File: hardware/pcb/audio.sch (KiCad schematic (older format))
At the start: 23 parts, among them J300 Conn_01x02, J301 AudioJack3_Ground_SwitchTR, U300 WM8960

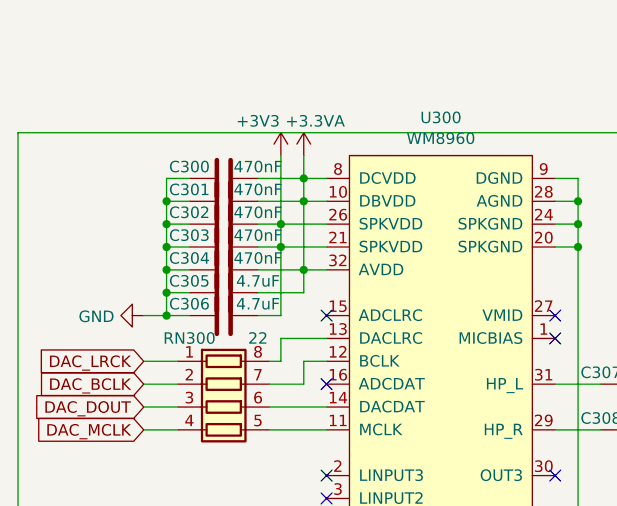
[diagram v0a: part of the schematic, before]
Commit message: vbh: pcb layout
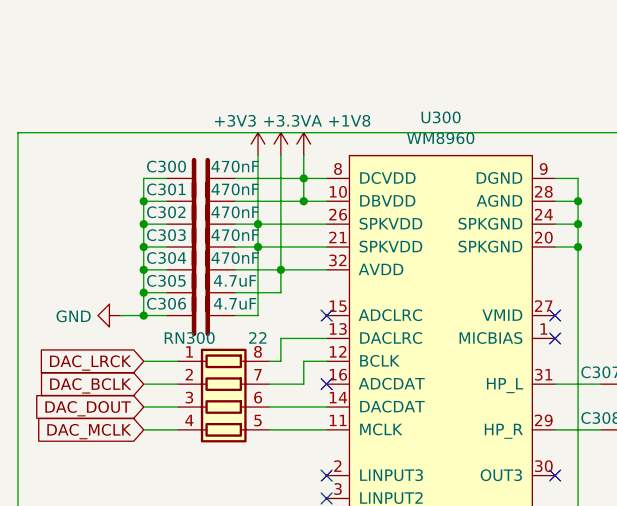
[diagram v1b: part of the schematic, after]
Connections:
- net +3.3VA: no longer C300.1, C301.1, U300.10 (DBVDD), U300.8 (DCVDD)
- new net +1V8: C300.1, C301.1, U300.10 (DBVDD), U300.8 (DCVDD)
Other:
- moved on the sheet: C300, C301, C302, C303, C304, C305, C306
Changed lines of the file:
@@
 L Device:C C?
 U 1 1 5EC1BEE7
-P 4600 3000
+P 4500 3000
 AR Path="/5E1291BC/5EC1BEE7" Ref="C?"  Part="1"
 AR Path="/5E1292AC/5EC1BEE7" Ref="C300"  Part="1"
-F 0 "C300" V 4550 2850 50  0000 C CNN
-F 1 "470nF" V 4550 3150 50  0000 C CNN
-F 2 "Capacitor_SMD:C_0402_1005Metric" H 4638 2850 50  0001 C CNN
-F 3 "~" H 4600 3000 50  0001 C CNN
-	1    4600 3000
+F 0 "C300" V 4450 2850 50  0000 C CNN
+F 1 "470nF" V 4450 3150 50  0000 C CNN
+F 2 "Capacitor_SMD:C_0402_1005Metric" H 4538 2850 50  0001 C CNN
+F 3 "~" H 4500 3000 50  0001 C CNN
+	1    4500 3000
 	0    1    1    0
 $EndComp
@@
 L Device:C C?
 U 1 1 5EC1BEED
-P 4600 3100
+P 4500 3100
 AR Path="/5E1291BC/5EC1BEED" Ref="C?"  Part="1"
 AR Path="/5E1292AC/5EC1BEED" Ref="C301"  Part="1"
-F 0 "C301" V 4550 2950 50  0000 C CNN
-F 1 "470nF" V 4550 3250 50  0000 C CNN
-F 2 "Capacitor_SMD:C_0402_1005Metric" H 4638 2950 50  0001 C CNN
-F 3 "~" H 4600 3100 50  0001 C CNN
-	1    4600 3100
+F 0 "C301" V 4450 2950 50  0000 C CNN
+F 1 "470nF" V 4450 3250 50  0000 C CNN
+F 2 "Capacitor_SMD:C_0402_1005Metric" H 4538 2950 50  0001 C CNN
+F 3 "~" H 4500 3100 50  0001 C CNN
+	1    4500 3100
 	0    1    1    0
 $EndComp
@@
 L Device:C C?
 U 1 1 5EC1BEF3
-P 4600 3500
+P 4500 3500
 AR Path="/5E1291BC/5EC1BEF3" Ref="C?"  Part="1"
 AR Path="/5E1292AC/5EC1BEF3" Ref="C305"  Part="1"
-F 0 "C305" V 4550 3350 50  0000 C CNN
-F 1 "4.7uF" V 4550 3650 50  0000 C CNN
-F 2 "Capacitor_SMD:C_0603_1608Metric" H 4638 3350 50  0001 C CNN
-F 3 "~" H 4600 3500 50  0001 C CNN
-	1    4600 3500
-	0    1    1    0
-$EndComp
-Wire Wire Line
-	4450 3000 4350 3000
-Wire Wire Line
-	4350 3000 4350 3100
-Wire Wire Line
-	4450 3100 4350 3100
-Connection ~ 4350 3100
-Wire Wire Line
-	4350 3100 4350 3200
-Wire Wire Line
-	4450 3200 4350 3200
-Connection ~ 4350 3200
+F 0 "C305" V 4450 3350 50  0000 C CNN
+F 1 "4.7uF" V 4450 3650 50  0000 C CNN
+F 2 "Capacitor_SMD:C_0603_1608Metric" H 4538 3350 50  0001 C CNN
+F 3 "~" H 4500 3500 50  0001 C CNN
+	1    4500 3500
+	0    1    1    0
+$EndComp
+Wire Wire Line
+	4350 3000 4250 3000
+Wire Wire Line
+	4250 3000 4250 3100
+Wire Wire Line
+	4350 3100 4250 3100
+Connection ~ 4250 3100
+Wire Wire Line
+	4250 3100 4250 3200
+Wire Wire Line
+	4350 3200 4250 3200
+Connection ~ 4250 3200
 $Comp
 L power:GND #PWR?
 U 1 1 5EC1BEFF
-P 4250 3600
+P 4150 3600
 AR Path="/5E1291BC/5EC1BEFF" Ref="#PWR?"  Part="1"
 AR Path="/5E1292AC/5EC1BEFF" Ref="#PWR055"  Part="1"
-F 0 "#PWR055" H 4250 3350 50  0001 C CNN
-F 1 "GND" V 4255 3472 50  0000 R CNN
-F 2 "" H 4250 3600 50  0001 C CNN
-F 3 "" H 4250 3600 50  0001 C CNN
-	1    4250 3600
+F 0 "#PWR055" H 4150 3350 50  0001 C CNN
+F 1 "GND" V 4155 3472 50  0000 R CNN
+F 2 "" H 4150 3600 50  0001 C CNN
+F 3 "" H 4150 3600 50  0001 C CNN
+	1    4150 3600
 	0    1    1    0
 $EndComp
@@
 L Device:C C?
 U 1 1 5EC1D61E
-P 4600 3600
+P 4500 3600
 AR Path="/5E1291BC/5EC1D61E" Ref="C?"  Part="1"
 AR Path="/5E1292AC/5EC1D61E" Ref="C306"  Part="1"
-F 0 "C306" V 4550 3450 50  0000 C CNN
-F 1 "4.7uF" V 4550 3750 50  0000 C CNN
-F 2 "Capacitor_SMD:C_0603_1608Metric" H 4638 3450 50  0001 C CNN
-F 3 "~" H 4600 3600 50  0001 C CNN
-	1    4600 3600
+F 0 "C306" V 4450 3450 50  0000 C CNN
+F 1 "4.7uF" V 4450 3750 50  0000 C CNN
+F 2 "Capacitor_SMD:C_0603_1608Metric" H 4538 3450 50  0001 C CNN
+F 3 "~" H 4500 3600 50  0001 C CNN
+	1    4500 3600
 	0    1    1    0
 $EndComp
@@
 L Device:C C?
 U 1 1 5EC1D831
-P 4600 3200
+P 4500 3200
 AR Path="/5E1291BC/5EC1D831" Ref="C?"  Part="1"
 AR Path="/5E1292AC/5EC1D831" Ref="C302"  Part="1"
-F 0 "C302" V 4550 3050 50  0000 C CNN
-F 1 "470nF" V 4550 3350 50  0000 C CNN
-F 2 "Capacitor_SMD:C_0402_1005Metric" H 4638 3050 50  0001 C CNN
-F 3 "~" H 4600 3200 50  0001 C CNN
-	1    4600 3200
+F 0 "C302" V 4450 3050 50  0000 C CNN
+F 1 "470nF" V 4450 3350 50  0000 C CNN
+F 2 "Capacitor_SMD:C_0402_1005Metric" H 4538 3050 50  0001 C CNN
+F 3 "~" H 4500 3200 50  0001 C CNN
+	1    4500 3200
 	0    1    1    0
 $EndComp
@@
 L Device:C C?
 U 1 1 5EC1D969
-P 4600 3300
+P 4500 3300
 AR Path="/5E1291BC/5EC1D969" Ref="C?"  Part="1"
 AR Path="/5E1292AC/5EC1D969" Ref="C303"  Part="1"
-F 0 "C303" V 4550 3150 50  0000 C CNN
-F 1 "470nF" V 4550 3450 50  0000 C CNN
-F 2 "Capacitor_SMD:C_0402_1005Metric" H 4638 3150 50  0001 C CNN
-F 3 "~" H 4600 3300 50  0001 C CNN
-	1    4600 3300
+F 0 "C303" V 4450 3150 50  0000 C CNN
+F 1 "470nF" V 4450 3450 50  0000 C CNN
+F 2 "Capacitor_SMD:C_0402_1005Metric" H 4538 3150 50  0001 C CNN
+F 3 "~" H 4500 3300 50  0001 C CNN
+	1    4500 3300
 	0    1    1    0
 $EndComp
@@
 L Device:C C?
 U 1 1 5EC1DAA6
-P 4600 3400
+P 4500 3400
 AR Path="/5E1291BC/5EC1DAA6" Ref="C?"  Part="1"
 AR Path="/5E1292AC/5EC1DAA6" Ref="C304"  Part="1"
-F 0 "C304" V 4550 3250 50  0000 C CNN
-F 1 "470nF" V 4550 3550 50  0000 C CNN
-F 2 "Capacitor_SMD:C_0402_1005Metric" H 4638 3250 50  0001 C CNN
-F 3 "~" H 4600 3400 50  0001 C CNN
-	1    4600 3400
-	0    1    1    0
-$EndComp
+F 0 "C304" V 4450 3250 50  0000 C CNN
+F 1 "470nF" V 4450 3550 50  0000 C CNN
+F 2 "Capacitor_SMD:C_0402_1005Metric" H 4538 3250 50  0001 C CNN
+F 3 "~" H 4500 3400 50  0001 C CNN
+	1    4500 3400
+	0    1    1    0
+$EndComp
+Wire Wire Line
+	4250 3600 4150 3600
+Wire Wire Line
+	4250 3200 4250 3300
 Wire Wire Line
 	4350 3600 4250 3600
-Wire Wire Line
-	4350 3200 4350 3300
-Wire Wire Line
-	4450 3600 4350 3600
-Connection ~ 4350 3600
-Wire Wire Line
-	4450 3300 4350 3300
-Connection ~ 4350 3300
-Wire Wire Line
-	4350 3300 4350 3400
-Wire Wire Line
-	4450 3400 4350 3400
-Connection ~ 4350 3400
-Wire Wire Line
-	4350 3400 4350 3500
-Wire Wire Line
-	4450 3500 4350 3500
-Connection ~ 4350 3500
-Wire Wire Line
-	4350 3500 4350 3600
+Connection ~ 4250 3600
+Wire Wire Line
+	4350 3300 4250 3300
+Connection ~ 4250 3300
+Wire Wire Line
+	4250 3300 4250 3400
+Wire Wire Line
+	4350 3400 4250 3400
+Connection ~ 4250 3400
+Wire Wire Line
+	4250 3400 4250 3500
+Wire Wire Line
+	4350 3500 4250 3500
+Connection ~ 4250 3500
+Wire Wire Line
+	4250 3500 4250 3600
 $Comp
 L power:+3V3 #PWR056
 U 1 1 5EC1ECB8
+P 4750 2900
+F 0 "#PWR056" H 4750 2750 50  0001 C CNN
+F 1 "+3V3" H 4650 3050 50  0000 C CNN
+F 2 "" H 4750 2900 50  0001 C CNN
+F 3 "" H 4750 2900 50  0001 C CNN
+	1    4750 2900
+	1    0    0    -1
+$EndComp
+$Comp
+L power:+3.3VA #PWR057
+U 1 1 5EC1F2E4
 P 4850 2900
-F 0 "#PWR056" H 4850 2750 50  0001 C CNN
-F 1 "+3V3" H 4750 3050 50  0000 C CNN
+F 0 "#PWR057" H 4850 2750 50  0001 C CNN
+F 1 "+3.3VA" H 4900 3050 50  0000 C CNN
 F 2 "" H 4850 2900 50  0001 C CNN
 F 3 "" H 4850 2900 50  0001 C CNN
@@
 	1    0    0    -1
 $EndComp
-$Comp
-L power:+3.3VA #PWR057
-U 1 1 5EC1F2E4
-P 4950 2900
-F 0 "#PWR057" H 4950 2750 50  0001 C CNN
-F 1 "+3.3VA" H 5000 3050 50  0000 C CNN
-F 2 "" H 4950 2900 50  0001 C CNN
-F 3 "" H 4950 2900 50  0001 C CNN
-	1    4950 2900
-	1    0    0    -1
-$EndComp
-Wire Wire Line
-	4950 3500 4950 3400
-Wire Wire Line
-	5050 3000 4950 3000
-Connection ~ 4950 3000
-Wire Wire Line
-	4950 3000 4950 2900
-Connection ~ 4950 3100
-Wire Wire Line
-	4950 3100 4950 3000
-Wire Wire Line
-	5050 3100 4950 3100
-Wire Wire Line
-	5050 3400 4950 3400
-Connection ~ 4950 3400
-Wire Wire Line
-	4950 3400 4950 3100
+Wire Wire Line
+	4850 3500 4850 3400
+Connection ~ 4850 3400
 $Comp
 L Device:R_Pack04 RN300
@@
 NoConn ~ 5050 4800
 Wire Wire Line
-	4750 3000 4950 3000
-Wire Wire Line
-	4750 3100 4950 3100
-Wire Wire Line
-	4850 2900 4850 3200
-Wire Wire Line
-	4850 3200 4750 3200
-Wire Wire Line
-	5050 3200 4850 3200
-Connection ~ 4850 3200
-Wire Wire Line
-	4750 3300 4850 3300
-Wire Wire Line
-	4850 3200 4850 3300
-Connection ~ 4850 3300
-Wire Wire Line
-	4850 3300 5050 3300
-Wire Wire Line
-	4750 3400 4950 3400
-Wire Wire Line
-	4750 3500 4950 3500
-Wire Wire Line
-	4750 3600 4850 3600
-Wire Wire Line
-	4850 3600 4850 3300
+	4750 2900 4750 3200
+Wire Wire Line
+	4750 3200 4650 3200
+Connection ~ 4750 3200
+Wire Wire Line
+	4650 3300 4750 3300
+Wire Wire Line
+	4750 3200 4750 3300
+Connection ~ 4750 3300
+Wire Wire Line
+	4650 3400 4850 3400
+Wire Wire Line
+	4650 3500 4850 3500
+Wire Wire Line
+	4650 3600 4750 3600
+Wire Wire Line
+	4750 3600 4750 3300
 Wire Wire Line
 	4800 4000 5050 4000
@@
 	8300 3600 8300 4400
 NoConn ~ 8100 3800
+Wire Wire Line
+	4850 2900 4850 3400
+Wire Wire Line
+	4650 3000 4950 3000
+Wire Wire Line
+	4750 3200 5050 3200
+Wire Wire Line
+	4750 3300 5050 3300
+Wire Wire Line
+	4850 3400 5050 3400
+$Comp
+L power:+1V8 #PWR?
+U 1 1 5E4F063D
+P 4950 2900
+F 0 "#PWR?" H 4950 2750 50  0001 C CNN
+F 1 "+1V8" H 5150 3050 50  0000 C CNN
+F 2 "" H 4950 2900 50  0001 C CNN
+F 3 "" H 4950 2900 50  0001 C CNN
+	1    4950 2900
+	1    0    0    -1
+$EndComp
+Wire Wire Line
+	4650 3100 4950 3100
+Wire Wire Line
+	4950 2900 4950 3000
+Connection ~ 4950 3000
+Wire Wire Line
+	4950 3000 5050 3000
+Wire Wire Line
+	4950 3000 4950 3100
+Connection ~ 4950 3100
+Wire Wire Line
+	4950 3100 5050 3100
 $EndSCHEMATC
